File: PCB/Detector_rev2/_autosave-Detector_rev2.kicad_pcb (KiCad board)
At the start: 2 copper layers, 51.4 x 44.4 mm, 56 parts, among them J1 Conn_01x03_Male, J2 Conn_01x03_Male, J3 Conn_Coaxial, U1 N-jfet_dual, U2 N-jfet_dual, U3 LM6171D, U4 LM6171D, U5 LT6657BHMS8-5, U6 LT1995, U7 DMMT3904

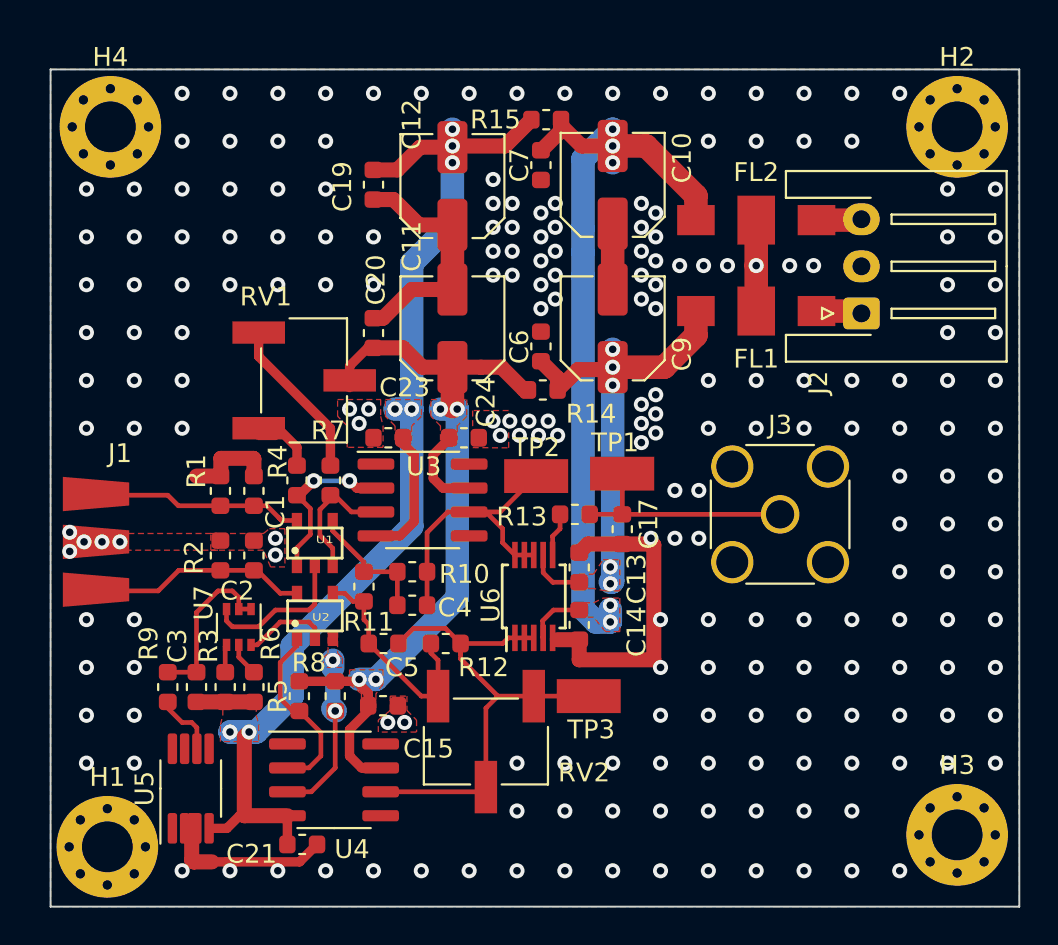
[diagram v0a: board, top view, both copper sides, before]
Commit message: garberdata output
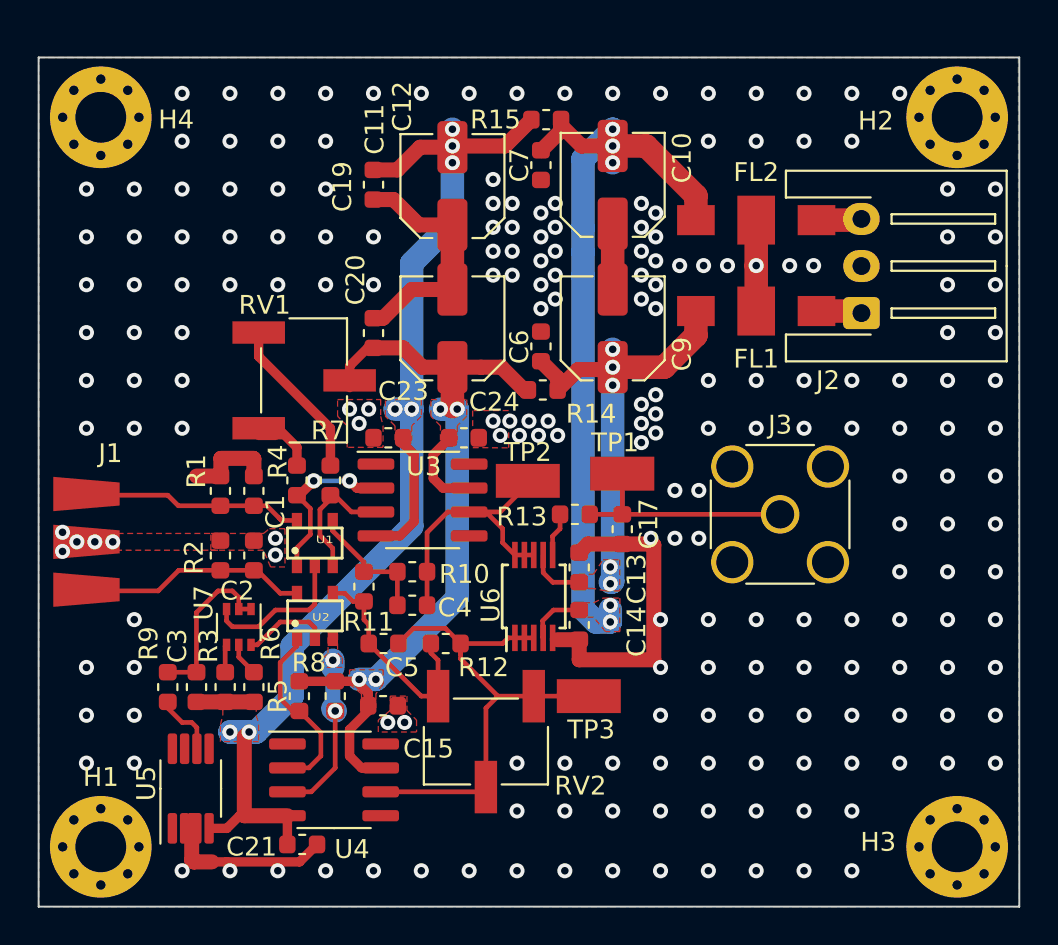
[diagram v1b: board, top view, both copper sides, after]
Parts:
- J2: footprint Connector_JST:JST_XH_S3B-XH-A-1_1x03_P2.50mm_Horizontal -> Detector_rev2:JST-XH_S3B
- moved J2 2.56 mm to (93.2, 53.6)
- moved H4 0.72 mm to (52.8, 45.7)
- moved H3 0.64 mm to (98.3, 84.5)
- moved TP2 0.51 mm to (75.5, 65.0)
- moved H2 0.51 mm to (98.3, 45.7)
- moved J1 0.51 mm to (52.1, 68.3)
- moved H1 0.35 mm to (52.8, 84.5)
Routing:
- net GND: vias 216 -> 215
- net (no net): vias 1 -> 0
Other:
- board size 51.4 x 44.4 mm -> 52.1 x 45.1 mm
- rule solder_mask_min_width: 0.25 -> 0.001
- rule trace_min: 0.2 -> 0.01
